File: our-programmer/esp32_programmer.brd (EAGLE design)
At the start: 66.2 x 35 mm, 59 parts, among them J16 10103592-0001LF-EK, Q1 MMBT3904_R1, Q2 MMBT3904_R1, U1 CP2102N-A02-GQFN24QFN24_CP210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, U2 AP2111H-3.3TRG1SOT-223_DIO-M, U3 NPN: BC817, U4 NPN: BC817, U5 NPN: BC817, U6 NPN: BC817

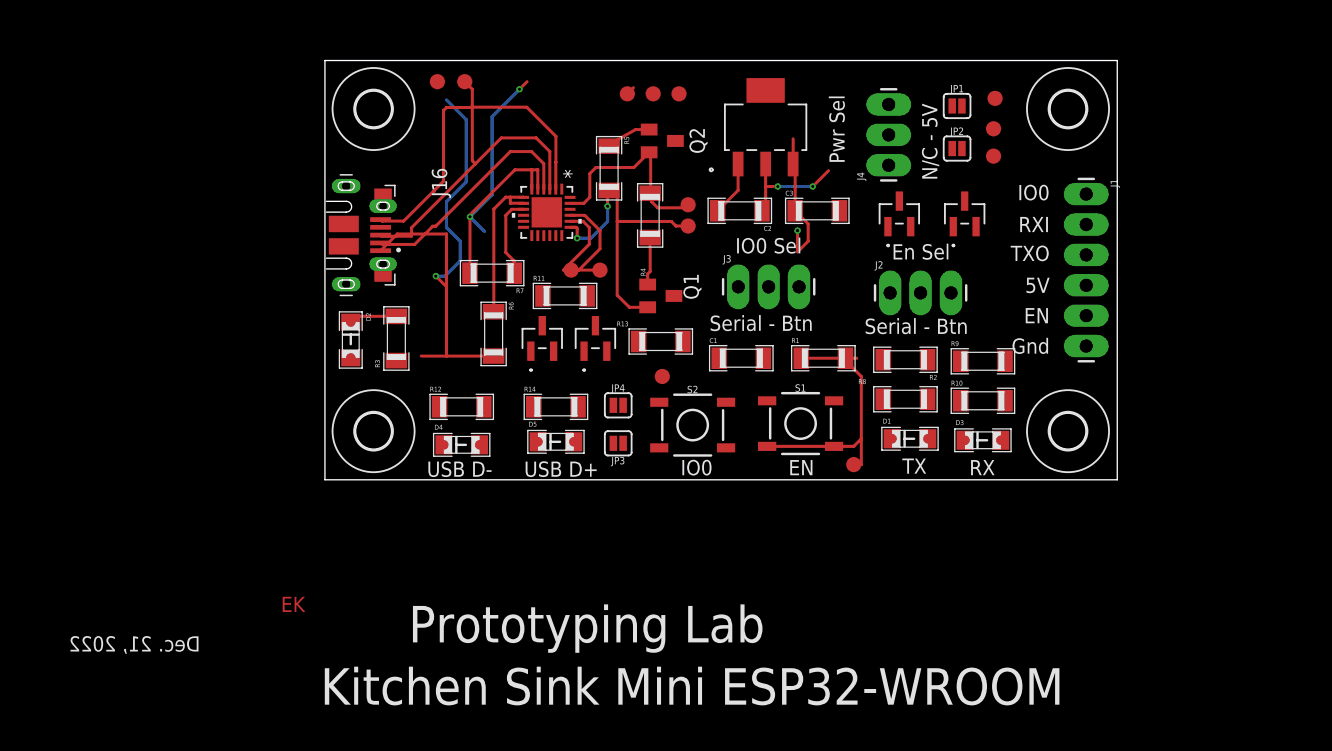
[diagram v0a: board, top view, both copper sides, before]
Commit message: Programmer board complete
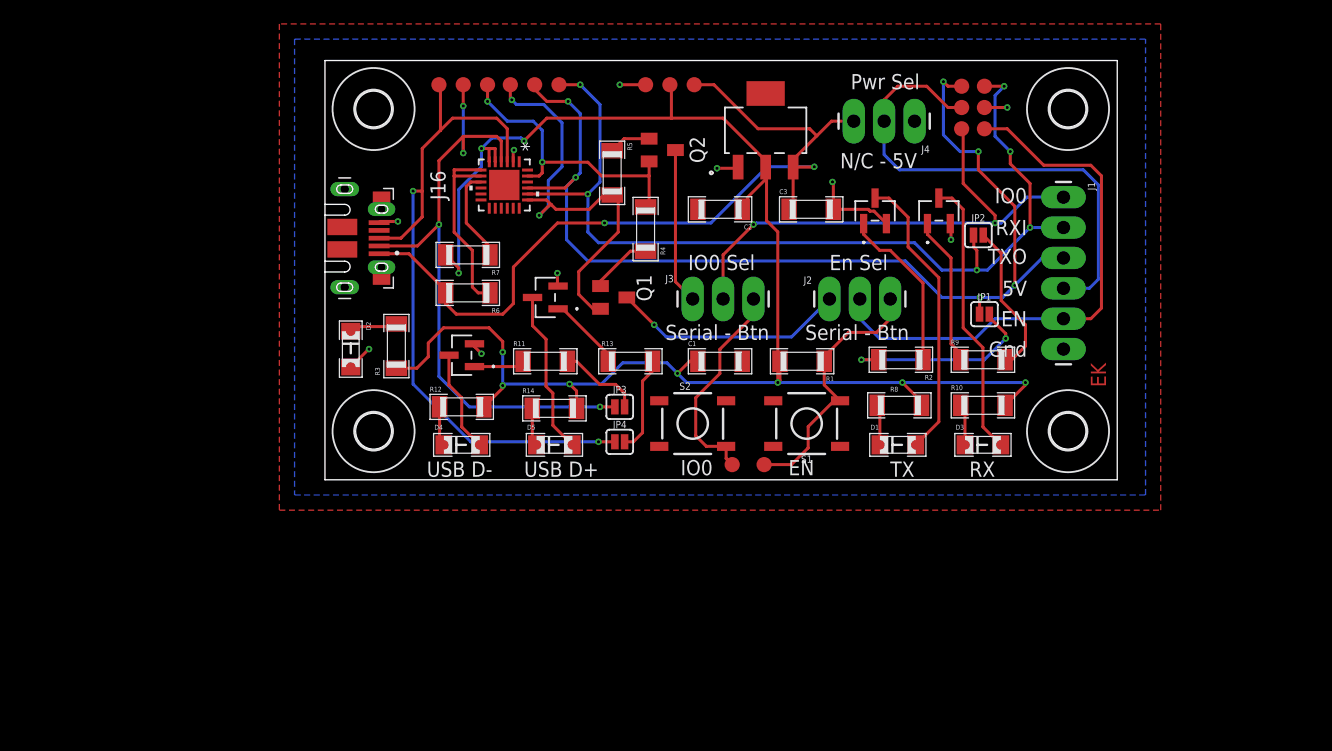
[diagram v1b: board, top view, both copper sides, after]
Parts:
- added TP1, TP2, TP3: TEST-POINT3X5, SparkFun-Connectors:PAD.03X.05
- moved TP62 19.5 mm to (13.6, 33.0)
- moved TP63 19.0 mm to (15.5, 33.0)
- moved JP1 17.5 mm to (55.1, 13.8)
- moved TP19 16.4 mm to (17.5, 33.0)
- moved TP20 15.5 mm to (19.6, 33.0)
- moved TP61 9.40 mm to (34.0, 1.27)
- moved TP60 7.49 mm to (36.7, 1.27)
- moved JP2 7.45 mm to (54.6, 20.4)
- moved U5 6.87 mm to (11.4, 10.4), turned to 90 degrees
- moved R11 5.71 mm to (18.4, 9.91)
- moved TP26 5.64 mm to (30.9, 33.0)
- moved U6 5.42 mm to (18.4, 15.2), turned to 90 degrees
- moved J2 5.11 mm to (42.2, 15.1)
- moved TP12 4.86 mm to (53.2, 31.1)
- moved J4 4.27 mm to (49.3, 30.0), turned to 180 degrees
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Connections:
- net GND1 renamed BLEP3
- net GND2 renamed BLEP4
- net GND3 renamed BLEP1
- net GND4 renamed BLEP2
- removed net N$2: C1.1
- removed net N$3: C1.2, S2.3
- net EN_SEL: now also TP2.P$1
- net GND: now also C1.2, S2.3, TP3.P$1
- net IO0_SEL: now also TP1.P$1
- net VCC: now also C1.1
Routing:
- net VCC: track 41.1 -> 142.5 mm, vias 4 -> 10
- net TX_SERIAL: track 8.85 -> 88.8 mm, vias 0 -> 6
- net RX_SERIAL: track 7.42 -> 80.8 mm, vias 0 -> 6
- net EN_SEL: track 0.00 -> 46.0 mm
- net IO0_SEL: track 0.00 -> 43.2 mm, vias 0 -> 2
- net PWR_SEL: track 0.00 -> 42.3 mm
- net USB_D-: track 19.3 -> 54.6 mm, vias 0 -> 4
- net USB_D+: track 28.8 -> 61.0 mm, vias 0 -> 2
- net BLEP3: track 0.00 -> 24.3 mm
- net BLEP4: track 0.00 -> 23.4 mm
- net EN_SERIAL: track 0.00 -> 19.6 mm, vias 0 -> 1
- net IO0_BUTTON: track 0.00 -> 18.1 mm
- net N$4: track 0.00 -> 16.9 mm, vias 0 -> 2
- net V_USB: track 54.3 -> 70.5 mm
- net N$13: track 0.00 -> 14.0 mm
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- added copper zone on layer 1, net GND
- added copper zone on layer 16, net GND
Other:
- board text added: ""Our ESP32 Programmer""
- board text added: "Dec. 23, 2022"
- board text removed: "Dec. 21, 2022"
- board text removed: "Kitchen Sink Mini ESP32-WROOM"
